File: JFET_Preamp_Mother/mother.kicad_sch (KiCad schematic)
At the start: 6 parts, among them J101 Conn_01x02

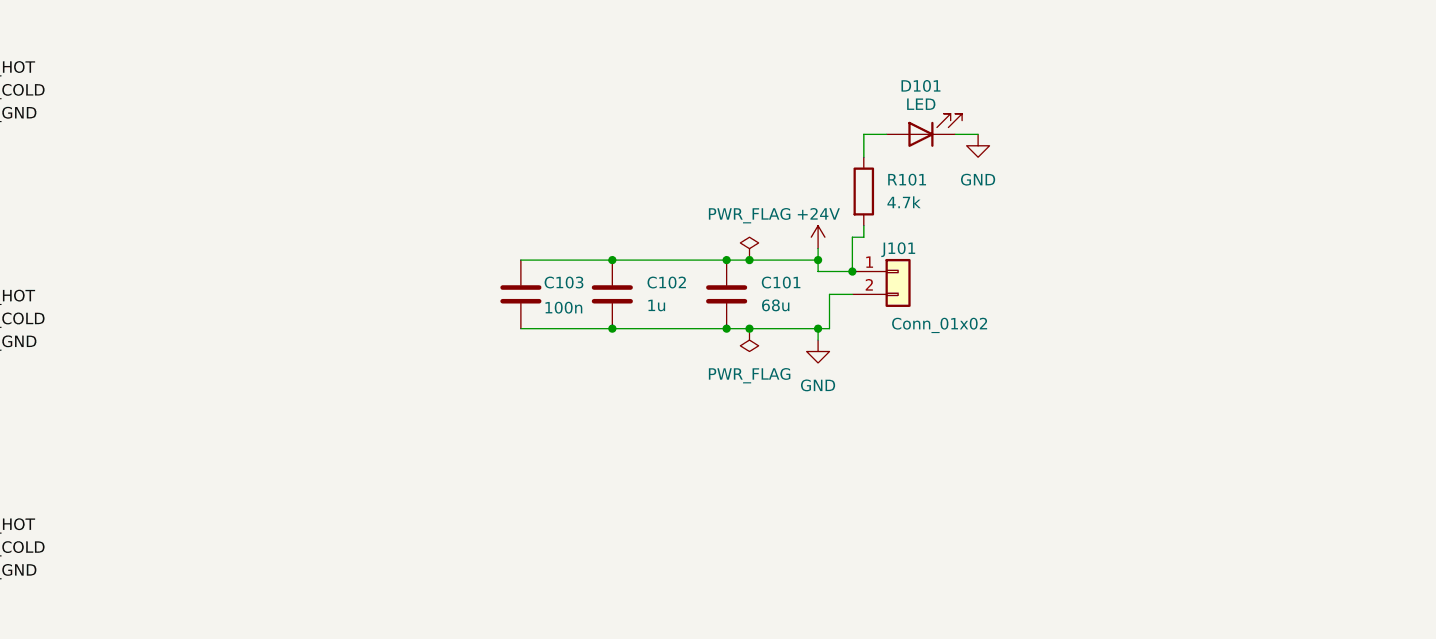
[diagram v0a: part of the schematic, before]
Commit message: motherboard .sch erc clean
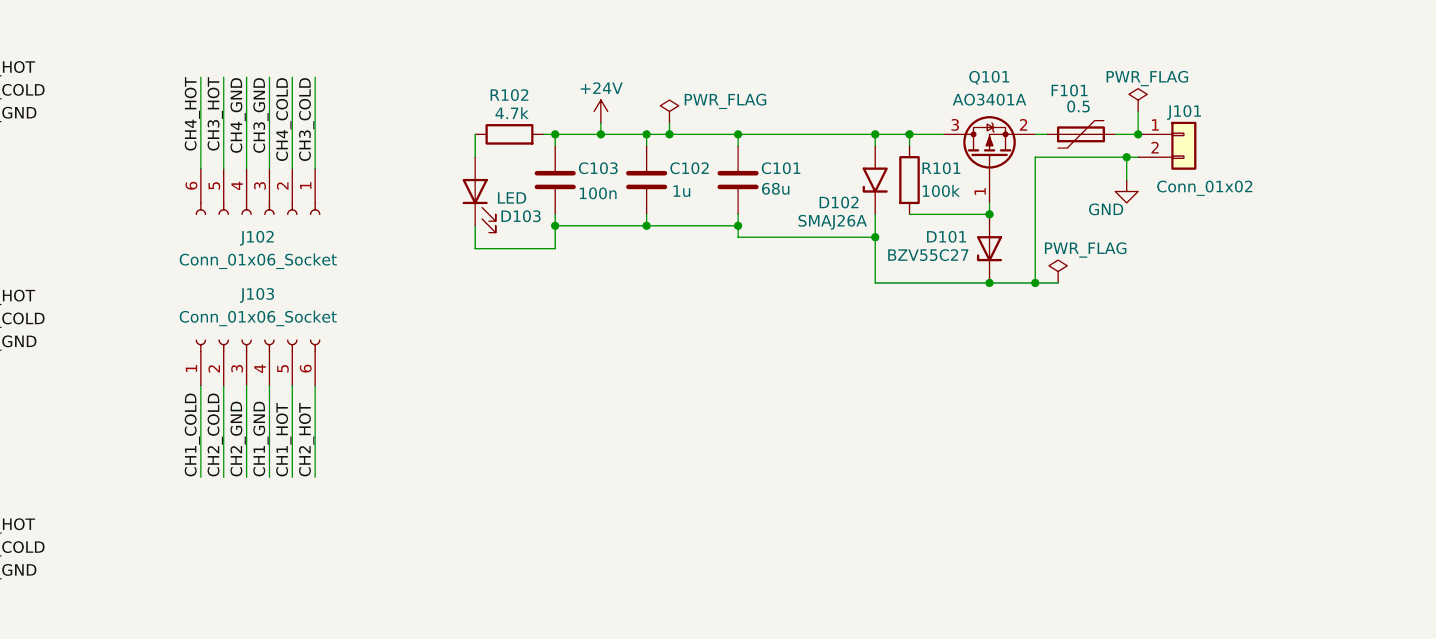
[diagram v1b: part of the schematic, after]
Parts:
- added D101: BZV55C27, Diode_SMD:D_MiniMELF, symbol Diode:BZV55C27
- added D102: SMAJ26A, Diode_SMD:D_SMA, symbol Diode:SMAJ26A
- added F101: 0.5, downloaded_footprints:FUSRB510W51L790T310H1370, symbol Device:Polyfuse
- added J102, J103: Conn_01x06_Socket, symbol Connector:Conn_01x06_Socket
- added Q101: AO3401A, Package_TO_SOT_SMD:SOT-23, symbol Transistor_FET:AO3401A
- added R102: 4.7k, symbol Device:R
- R101: value 4.7k -> 100k; footprint Resistor_SMD:R_0603_1608Metric -> (none)
- renumbered D101 to D103
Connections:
- net +24V: now also R101.1, D102.2 (A2), Q101.3 (D), R102.2; no longer J101.1 (Pin_1), R101.2
- net CH1_COLD: now also J103.1 (Pin_1)
- net CH1_GND: now also J103.4 (Pin_4)
- net CH1_HOT: now also J103.5 (Pin_5)
- net CH2_COLD: now also J103.2 (Pin_2)
- net CH2_GND: now also J103.3 (Pin_3)
- net CH2_HOT: now also J103.6 (Pin_6)
- net CH3_COLD: now also J102.1 (Pin_1)
- net CH3_GND: now also J102.3 (Pin_3)
- net CH3_HOT: now also J102.5 (Pin_5)
- net CH4_COLD: now also J102.2 (Pin_2)
- net CH4_GND: now also J102.4 (Pin_4)
- net CH4_HOT: now also J102.6 (Pin_6)
- net GND: now also D101.1 (K), D102.1 (A1)
- net at D103.2 (A): now also R102.1; no longer R101.1
- new net: D101.2 (A), Q101.1 (G), R101.2
- new net: F101.1, Q101.2 (S)
- new net: F101.2, J101.1 (Pin_1)
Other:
- moved on the sheet: C101, C102, C103, D103, J101
